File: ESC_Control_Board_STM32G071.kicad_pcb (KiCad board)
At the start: 2 copper layers, 0 parts

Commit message: Layout updates
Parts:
- added C1: 4u7, Capacitor_SMD:C_0603_1608Metric, F.Cu at (138.6, 25.1)
- added C10: 4u7, Capacitor_SMD:C_0603_1608Metric, F.Cu at (111.0, 71.3)
- added C11: 100n, Capacitor_SMD:C_0805_2012Metric, F.Cu at (154.7, 76.0)
- added C12: 100n, Capacitor_SMD:C_0603_1608Metric, F.Cu at (114.8, 56.5)
- added C14: 100n, Capacitor_SMD:C_0603_1608Metric, F.Cu at (111.0, 64.5)
- added C15: 47u, Capacitor_SMD:C_1210_3225Metric, F.Cu at (128.8, 28.4)
- added C16: 47u, Capacitor_SMD:C_1210_3225Metric, F.Cu at (111.8, 62.0)
- added C17: 100n, Capacitor_SMD:C_0603_1608Metric, F.Cu at (154.1, 66.2)
- added C18: 10u, Capacitor_SMD:C_0603_1608Metric, F.Cu at (152.5, 66.2)
- added C19: 47u, Capacitor_SMD:C_1210_3225Metric, F.Cu at (144.4, 59.3)
- added C2: 4u7, Capacitor_SMD:C_0603_1608Metric, F.Cu at (128.8, 25.0)
- added C20: 47u, Capacitor_SMD:C_1210_3225Metric, F.Cu at (147.7, 59.3)
- added C21: 2n2, Capacitor_SMD:C_0603_1608Metric, F.Cu at (119.0, 60.7)
- added C22: 2n2, Capacitor_SMD:C_0603_1608Metric, F.Cu at (117.6, 51.0)
- added C23: 2n2, Capacitor_SMD:C_0603_1608Metric, F.Cu at (118.1, 56.5)
- added C24: 4u7, Capacitor_SMD:C_0603_1608Metric, F.Cu at (147.7, 54.5)
- added C25: 4u7, Capacitor_SMD:C_0603_1608Metric, F.Cu at (139.7, 28.4)
- added C3: 4u7, Capacitor_SMD:C_0603_1608Metric, F.Cu at (143.1, 25.0)
- added C4: 4u7, Capacitor_SMD:C_0603_1608Metric, F.Cu at (123.2, 25.1)
- added C5: 100n, Capacitor_SMD:C_0603_1608Metric, F.Cu at (119.8, 54.5)
- added C6: 4u7, Capacitor_SMD:C_0603_1608Metric, F.Cu at (146.2, 72.0)
- added C7: 4u7, Capacitor_SMD:C_0603_1608Metric, F.Cu at (135.0, 72.0)
- added C8: 4u7, Capacitor_SMD:C_0603_1608Metric, F.Cu at (124.0, 71.8)
- added C9: 4u7, Capacitor_SMD:C_0603_1608Metric, F.Cu at (133.8, 32.2)
- added D1: ES1JFL, Diode_SMD:D_SOD-123F, F.Cu at (145.4, 67.4)
- added D2: ES1JFL, Diode_SMD:D_SOD-123F, F.Cu at (134.3, 67.4)
- added D3: ES1JFL, Diode_SMD:D_SOD-123F, F.Cu at (123.3, 67.3)
- added D4: 13V, Diode_SMD:D_SOD-523, F.Cu at (146.2, 70.4)
- added D5: 13V, Diode_SMD:D_SOD-523, F.Cu at (135.0, 70.5)
- added D6: 13V, Diode_SMD:D_SOD-523, F.Cu at (124.0, 70.3)
- added D7: ES1JFL, Diode_SMD:D_SOD-123F, F.Cu at (157.0, 76.1)
- added D8: ES1JFL, Diode_SMD:D_SOD-123F, F.Cu at (149.8, 65.5)
- added IC1: ISO1050DUBR, MAG_ESC:SOP254P1040X485-8N, F.Cu at (139.9, 19.2)
- added IC2: ISO1050DUBR, MAG_ESC:SOP254P1040X485-8N, F.Cu at (127.6, 19.2)
- added IC3: STM32G071RBT6, MAG_ESC:QFP50P1200X1200X160-64N, F.Cu at (127.3, 55.0)
- added IC4: AZ1117CR-3.3TRG1, MAG_ESC:AZ1117CR33TRG1, F.Cu at (113.2, 67.9)
- added IC5: ISO1540QDRQ1, MAG_ESC:SOIC127P600X175-8N, F.Cu at (145.7, 50.9)
- added IC6: INA240A2PW, MAG_Current_Sense_Amplifiers:SOP65P640X120-8N, F.Cu at (141.8, 31.1)
- added J2: Conn_01x03, MAG_Connectors:PWM_PADS, F.Cu at (152.1, 51.6)
- added J3: Conn_01x04, Connector_Molex:Molex_PicoBlade_53261-0471_1x04-1MP_P1.25mm_Horizontal, F.Cu at (150.1, 18.9)
- added J4: Conn_01x04, Connector_Molex:Molex_PicoBlade_53261-0471_1x04-1MP_P1.25mm_Horizontal, F.Cu at (117.3, 18.9)
- added J5: Conn_01x02, Connector_Molex:Molex_PicoBlade_53261-0271_1x02-1MP_P1.25mm_Horizontal, F.Cu at (150.1, 31.2)
- added J6: Conn_01x15, Connector_PinHeader_2.00mm:PinHeader_1x15_P2.00mm_Vertical, F.Cu at (145.7, 79.9)
- added J7: TC6NL_SWD, MAG_ESC:TC2030IDC, F.Cu at (138.1, 56.8)
- added L1: 1m, Inductor_SMD:L_7.3x7.3_H4.5, F.Cu at (153.8, 59.2)
- added PS1: AZ1117CR-5.0TRG1, MAG_LDO_Regulators:AZ1117CR33TRG1, F.Cu at (133.8, 26.5)
- added R1: 20R, Resistor_SMD:R_0603_1608Metric, F.Cu at (139.2, 72.0)
- added R10: 5R1, Resistor_SMD:R_0805_2012Metric, F.Cu at (127.8, 76.7)
- added R11: 5R1, Resistor_SMD:R_0805_2012Metric, F.Cu at (120.3, 75.9)
- added R12: 5R1, Resistor_SMD:R_0805_2012Metric, F.Cu at (113.3, 78.5)
- added R13: 100k, Resistor_SMD:R_0805_2012Metric, F.Cu at (152.6, 76.0)
- added R14: 2k, Resistor_SMD:R_0603_1608Metric, F.Cu at (113.3, 56.5)
- added R15: 2k, Resistor_SMD:R_0603_1608Metric, F.Cu at (155.7, 66.2)
- added R16: 13k3, Resistor_SMD:R_0603_1608Metric, F.Cu at (149.7, 69.7)
- added R17: 200k, Resistor_SMD:R_0805_2012Metric, F.Cu at (125.5, 67.3)
- added R18: 2k7, Resistor_SMD:R_0603_1608Metric, F.Cu at (117.5, 60.7)
- added R19: 200k, Resistor_SMD:R_0805_2012Metric, F.Cu at (136.5, 67.4)
- added R2: 20R, Resistor_SMD:R_0603_1608Metric, F.Cu at (126.8, 72.6)
- added R20: 2k7, Resistor_SMD:R_0603_1608Metric, F.Cu at (119.1, 51.0)
- added R21: 200k, Resistor_SMD:R_0805_2012Metric, F.Cu at (147.6, 67.4)
- added R22: 2k7, Resistor_SMD:R_0603_1608Metric, F.Cu at (116.6, 56.5)
- added R23: 510R, Resistor_SMD:R_0603_1608Metric, F.Cu at (150.3, 51.6)
- added R24: 510R, Resistor_SMD:R_0603_1608Metric, F.Cu at (143.5, 54.5)
- added R3: 20R, Resistor_SMD:R_0603_1608Metric, F.Cu at (116.6, 72.0)
- added R4: 20R, Resistor_SMD:R_0603_1608Metric, F.Cu at (142.8, 72.0)
- added R5: 20R, Resistor_SMD:R_0603_1608Metric, F.Cu at (130.0, 72.0)
- added R6: 20R, Resistor_SMD:R_0603_1608Metric, F.Cu at (119.8, 72.0)
- added R7: 5R1, Resistor_SMD:R_0805_2012Metric, F.Cu at (144.4, 76.7)
- added R8: 5R1, Resistor_SMD:R_0805_2012Metric, F.Cu at (137.7, 76.7)
- added R9: 5R1, Resistor_SMD:R_0805_2012Metric, F.Cu at (135.3, 76.7)
- added U1: L6498DTR, MAG_Gate_Drivers:SOT127P600X175-8N, F.Cu at (141.3, 67.3)
- added U10: LNK306DN-TL, MAG_Switching_Regulators:SOIC127P600X175-8N, F.Cu at (154.3, 71.1)
- added U2: L6498DTR, MAG_Gate_Drivers:SOT127P600X175-8N, F.Cu at (130.2, 67.3)
- added U3: L6498DTR, MAG_Gate_Drivers:SOT127P600X175-8N, F.Cu at (119.2, 67.3)
- added U4: ZXGD3006E6QTA, MAG_Gate_Drivers:SOT95P285X140-6N, F.Cu at (147.9, 75.9)
- added U5: ZXGD3006E6QTA, MAG_Gate_Drivers:SOT95P285X140-6N, F.Cu at (141.2, 75.9)
- added U6: ZXGD3006E6QTA, MAG_Gate_Drivers:SOT95P285X140-6N, F.Cu at (131.9, 76.0)
- added U7: ZXGD3006E6QTA, MAG_Gate_Drivers:SOT95P285X140-6N, F.Cu at (123.7, 76.1)
- added U8: ZXGD3006E6QTA, MAG_Gate_Drivers:SOT95P285X140-6N, F.Cu at (117.2, 75.9)
- added U9: ZXGD3006E6QTA, MAG_Gate_Drivers:SOT95P285X140-6N, F.Cu at (113.3, 74.5)
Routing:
- net /MCU/VOLT_SENSE: track 0.00 -> 64.7 mm, vias 0 -> 3
- net +12V: track 0.00 -> 57.1 mm, vias 0 -> 29
- net /MCU/USART1_TX: track 0.00 -> 51.7 mm, vias 0 -> 2
- net /MCU/USART1_RX: track 0.00 -> 48.7 mm, vias 0 -> 2
- net /MCU/pU_COMP: track 0.00 -> 47.5 mm, vias 0 -> 2
- net /MCU/pV_COMP: track 0.00 -> 38.8 mm, vias 0 -> 2
- net /MCU/CURR_SENSE: track 0.00 -> 38.6 mm, vias 0 -> 2
- net /MCU/USART2_TX: track 0.00 -> 35.0 mm, vias 0 -> 2
- net /MCU/USART2_RX: track 0.00 -> 33.0 mm, vias 0 -> 2
- net /BEMF_Feedback/pW: track 0.00 -> 28.9 mm, vias 0 -> 4
- net /MCU/INPUT_PIN: track 0.00 -> 27.6 mm
- net /BEMF_Feedback/pU: track 0.00 -> 27.6 mm, vias 0 -> 5
- net +5V: track 0.00 -> 24.4 mm, vias 0 -> 2
- net /BEMF_Feedback/pV: track 0.00 -> 20.2 mm, vias 0 -> 4
- net Net-(C17-Pad2): track 0.00 -> 20.1 mm
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- added copper zone on B.Cu, net +12V
- added copper zone on F.Cu, net +12V
- added copper zone on F.Cu, net +3V3
- added copper zone on In3.Cu, net +3V3
- added copper zone on In3.Cu, net +5V
- added copper zone on F.Cu, net /BEMF_Feedback/pU
- added copper zone on F.Cu, net /BEMF_Feedback/pV
- added copper zone on F.Cu, net /BEMF_Feedback/pW
- added copper zone on F.Cu, net /Gate_Drive/U_L
- added copper zone on F.Cu, net /Gate_Drive/V_H
- added copper zone on F.Cu, net /Gate_Drive/V_L
- added copper zone on F.Cu, net /Gate_Drive/W_H
- added copper zone on F.Cu, net /Gate_Drive/W_L
- added copper zone on B.Cu, net /Power_Supplies/VBATT
- added copper zone on F.Cu, net /Power_Supplies/VBATT
- added copper zone on F.Cu, net GND
- added copper zone on In1.Cu, net GND
- added copper zone on In4.Cu, net GND
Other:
- board outline added: 50 x 67 mm
- copper layers 2 -> 6

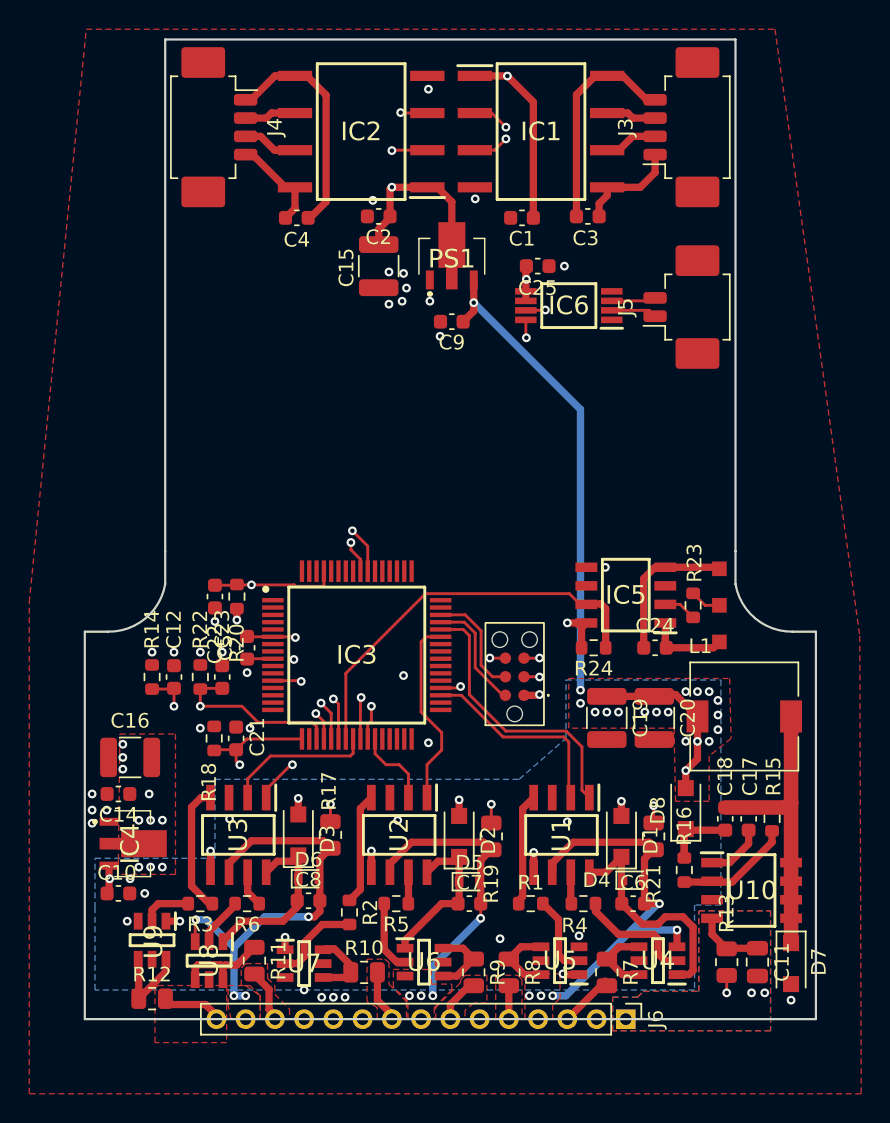
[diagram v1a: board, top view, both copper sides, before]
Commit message: Updates for review
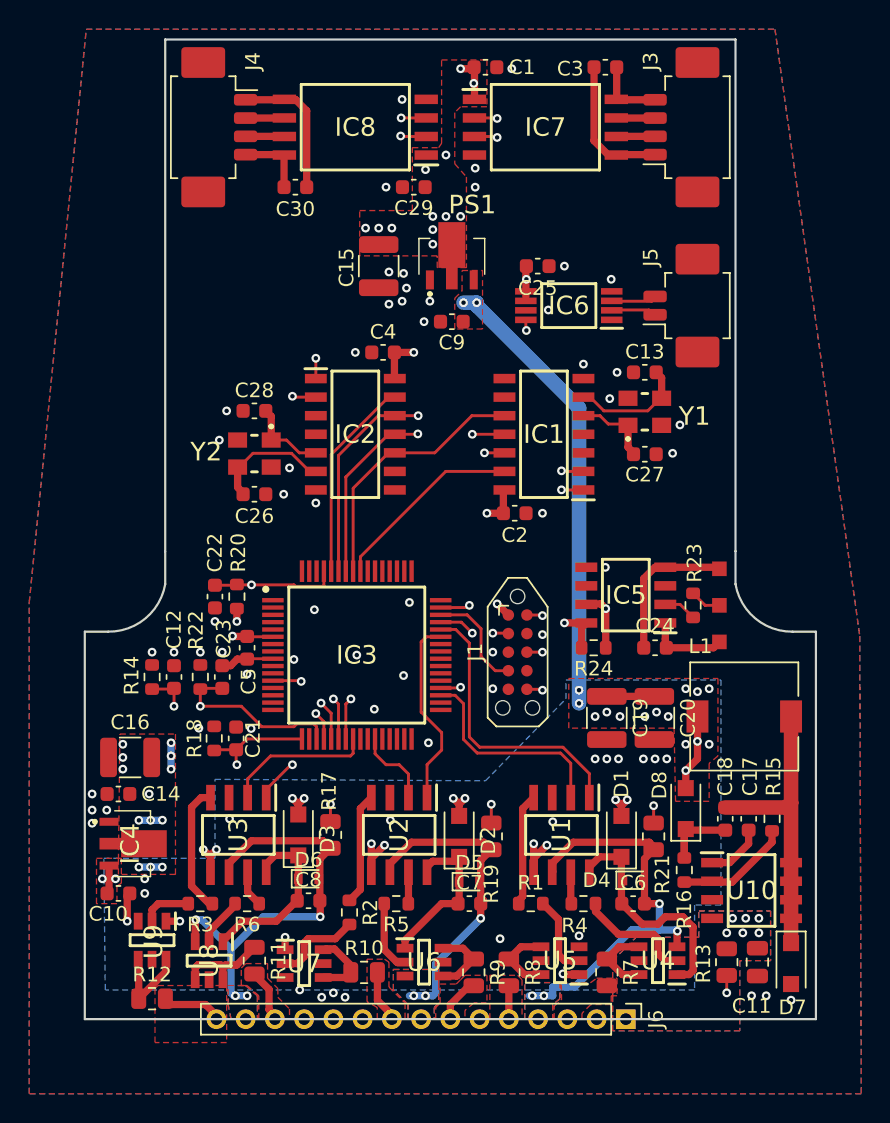
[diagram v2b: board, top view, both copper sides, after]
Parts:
- removed J7: TC6NL_SWD, MAG_ESC:TC2030IDC
- added C13: 12p, Capacitor_SMD:C_0603_1608Metric, F.Cu at (147.0, 35.7)
- added C26: 12p, Capacitor_SMD:C_0603_1608Metric, F.Cu at (120.3, 44.0)
- added C27: 12p, Capacitor_SMD:C_0603_1608Metric, F.Cu at (147.0, 41.3)
- added C28: 12p, Capacitor_SMD:C_0603_1608Metric, F.Cu at (120.3, 38.3)
- added C29: 4u7, Capacitor_SMD:C_0603_1608Metric, F.Cu at (131.2, 23.0)
- added C30: 4u7, Capacitor_SMD:C_0603_1608Metric, F.Cu at (123.1, 23.0)
- added IC7: ADM3050EBRIZ, MAG_CAN_Transceivers:SOIC127P1031X265-8N, F.Cu at (140.2, 18.9)
- added IC8: ADM3050EBRIZ, MAG_CAN_Transceivers:SOIC127P1031X265-8N, F.Cu at (127.2, 18.9)
- added J1: Conn_ARM_JTAG_SWD_10, Connector:Tag-Connect_TC2050-IDC-NL_2x05_P1.27mm_Vertical_with_bottom_clip, F.Cu at (138.3, 54.8)
- added Y1: ABM8-20.000MHZ-10-B1U-T, MAG_Crystals:ABM810000MHZ12D2W, F.Cu at (147.0, 38.4)
- added Y2: ABM8-20.000MHZ-10-B1U-T, MAG_Crystals:ABM810000MHZ12D2W, F.Cu at (120.3, 41.2)
- IC1, IC2: value ISO1050DUBR -> MCP2518FDT-E_SL; footprint MAG_ESC:SOP254P1040X485-8N -> MAG_CAN_Transceivers:SOIC127P600X175-14N
- moved C2 22.3 mm to (138.1, 45.3), turned to 0 degrees
- moved IC2 20.7 mm to (127.2, 39.9), turned to 0 degrees
- moved IC1 20.7 mm to (140.1, 39.9), turned to 180 degrees
- moved C4 10.9 mm to (129.1, 34.3), turned to 180 degrees
- moved C1 10.6 mm to (136.1, 14.8), turned to 0 degrees
- moved C3 10.3 mm to (144.3, 14.8), turned to 180 degrees
- moved J5 0.10 mm to (150.1, 31.1)
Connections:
- C11 pad 1: /Power_Supplies/VBATT -> VBATT
- C2 pad 1: +5V -> +3V3
- C4 pad 1: /CAN/+5V_ISO2 -> +3V3
- C4 pad 2: /CAN/GND_ISO2 -> GND
- IC1 pad 1: +5V -> Net-(IC1-Pad1)
- IC1 pad 2: /MCU/USART1_RX -> Net-(IC1-Pad2)
- IC1 pad 3: /MCU/USART1_TX -> unconnected-(IC1-Pad3)
- IC1 pad 4: GND -> unconnected-(IC1-Pad4)
- IC1 pad 5: /CAN/GND_ISO1 -> Net-(C27-Pad1)
- IC1 pad 6: /CAN/CAN_L1 -> Net-(C13-Pad1)
- IC1 pad 7: /CAN/CAN_H1 -> GND
- IC1 pad 8: /CAN/+5V_ISO1 -> unconnected-(IC1-Pad8)
- IC2 pad 1: +5V -> Net-(IC2-Pad1)
- IC2 pad 2: /MCU/USART2_RX -> Net-(IC2-Pad2)
- IC2 pad 3: /MCU/USART2_TX -> unconnected-(IC2-Pad3)
- IC2 pad 4: GND -> unconnected-(IC2-Pad4)
- IC2 pad 5: /CAN/GND_ISO2 -> Net-(C28-Pad1)
- IC2 pad 6: /CAN/CAN_L2 -> Net-(C26-Pad1)
- IC2 pad 7: /CAN/CAN_H2 -> GND
- IC2 pad 8: /CAN/+5V_ISO2 -> unconnected-(IC2-Pad8)
- IC3 pad 13: unconnected-(IC3-Pad13) -> /MCU/PC0
- IC3 pad 14: unconnected-(IC3-Pad14) -> /MCU/PC1
- IC3 pad 15: unconnected-(IC3-Pad15) -> /MCU/PC2
- IC3 pad 25: /MCU/USART1_TX -> unconnected-(IC3-Pad25)
- IC3 pad 26: /MCU/USART1_RX -> unconnected-(IC3-Pad26)
- IC3 pad 47: unconnected-(IC3-Pad47) -> /MCU/TDI
- IC3 pad 54: /MCU/CAN2_EN -> unconnected-(IC3-Pad54)
- IC3 pad 55: /MCU/USART2_TX -> unconnected-(IC3-Pad55)
- IC3 pad 56: /MCU/USART2_RX -> /MCU/CAN1_CS
- IC3 pad 57: unconnected-(IC3-Pad57) -> /MCU/SCK
- IC3 pad 58: unconnected-(IC3-Pad58) -> /MCU/MISO
- IC3 pad 59: unconnected-(IC3-Pad59) -> /MCU/MOSI
- IC3 pad 60: unconnected-(IC3-Pad60) -> /MCU/CAN2_CS
- R13 pad 1: /Power_Supplies/VBATT -> VBATT
- U10 pad 4: /Power_Supplies/VBATT -> VBATT
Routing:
- net /MCU/USART1_TX: track 51.7 -> 0.00 mm, vias 2 -> 0
- net /MCU/USART1_RX: track 48.7 -> 0.00 mm, vias 2 -> 0
- net /MCU/USART2_TX: track 35.0 -> 0.00 mm, vias 2 -> 0
- net /MCU/USART2_RX: track 33.0 -> 0.00 mm, vias 2 -> 0
- net Net-(IC1-Pad1): track 0.00 -> 30.8 mm, vias 0 -> 2
- net Net-(IC1-Pad2): track 0.00 -> 27.7 mm, vias 0 -> 2
- net Net-(IC2-Pad2): track 0.00 -> 25.5 mm, vias 0 -> 2
- net /MCU/MOSI: track 0.00 -> 22.5 mm, vias 0 -> 2
- net +5V: track 24.4 -> 3.03 mm, vias 2 -> 12
- net Net-(IC2-Pad1): track 0.00 -> 21.1 mm, vias 0 -> 2
- net /MCU/MISO: track 0.00 -> 18.6 mm, vias 0 -> 2
- net /MCU/SCK: track 0.00 -> 18.1 mm
- net /MCU/CAN2_CS: track 0.00 -> 14.0 mm
- net /MCU/CAN1_CS: track 0.00 -> 13.3 mm
- net +3V3: track 9.41 -> 19.9 mm, vias 11 -> 16
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- added copper zone on F.Cu, net +5V
- added copper zone on B.Cu, net /BEMF_Feedback/pU
- added copper zone on B.Cu, net /BEMF_Feedback/pV
- added copper zone on B.Cu, net /BEMF_Feedback/pW
- added copper zone on F.Cu, net /Gate_Drive/U_H
- added copper zone on B.Cu, net GND
- added copper zone on B.Cu, net VBATT
- added copper zone on F.Cu, net VBATT
- removed copper zone on B.Cu, net /Power_Supplies/VBATT
- removed copper zone on F.Cu, net /Power_Supplies/VBATT
